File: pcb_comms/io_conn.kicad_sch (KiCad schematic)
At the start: 15 parts, among them IC1 CP2102N-A02-GQFN28, J1 Conn_01x06_Pin, J2 USB_B_Micro

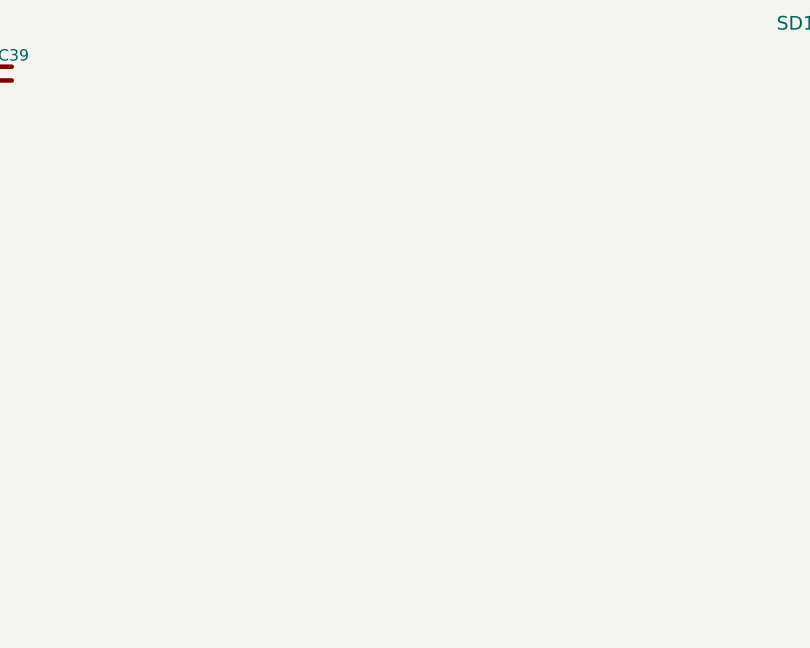
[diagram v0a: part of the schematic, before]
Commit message: Update GPS
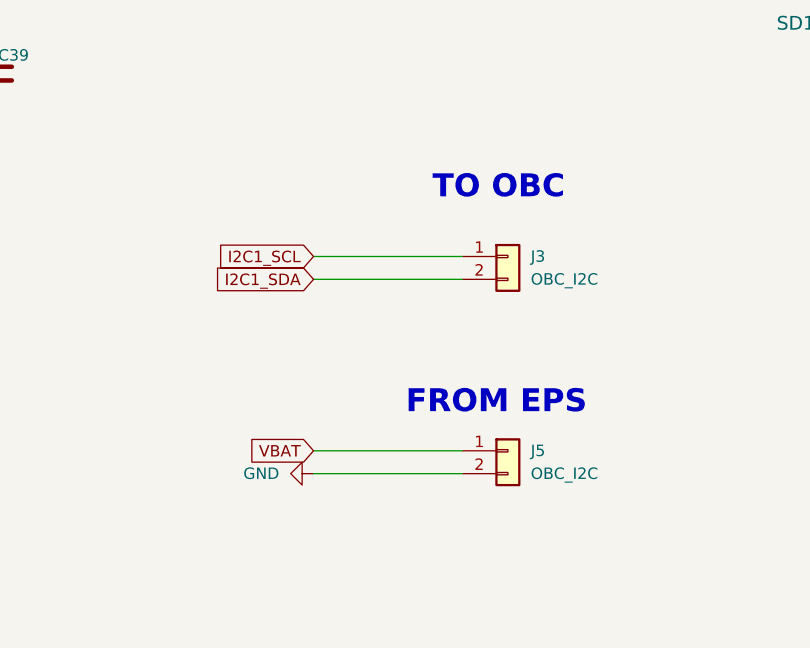
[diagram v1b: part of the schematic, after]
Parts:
- added J3, J5: OBC_I2C, symbol Connector_Generic:Conn_01x02
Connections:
- net GND: now also J5.2 (Pin_2)
- new net I2C1_SCL: J3.1 (Pin_1)
- new net I2C1_SDA: J3.2 (Pin_2)
- new net VBAT: J5.1 (Pin_1)
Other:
- note added: "FROM EPS"
- note added: "TO OBC"
